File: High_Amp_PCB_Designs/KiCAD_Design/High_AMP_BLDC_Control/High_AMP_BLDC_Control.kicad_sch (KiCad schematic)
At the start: 4 parts

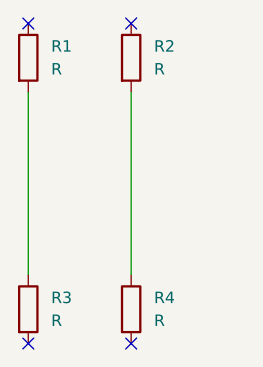
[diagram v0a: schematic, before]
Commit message: :construction: Python script ongoing.
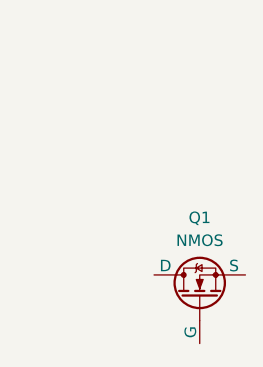
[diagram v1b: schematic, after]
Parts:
- removed R1, R2, R3, R4: R, Resistor_SMD:R_0201_0603Metric_Pad0.64x0.40mm_HandSolder, symbol Device:R
- added Q1: NMOS, FOOTPRINT:MOSFET_CSD19531Q5A, symbol Simulation_SPICE:NMOS
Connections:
- no-connect marks 4 -> 0
